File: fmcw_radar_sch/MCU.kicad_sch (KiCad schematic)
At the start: 39 parts, among them J1 2x5 1.27mm, J2 Conn_01x04_Pin, J3 Conn_01x07_Pin, J4 Conn_01x05_Pin, J5 Conn_01x04_Pin, J6 Conn_01x03_Pin, J7 Conn_01x04_Pin, SW1 SW_SPDT, U1 STM32F103C8T6, Y1 HC-49US 16MHZ THT

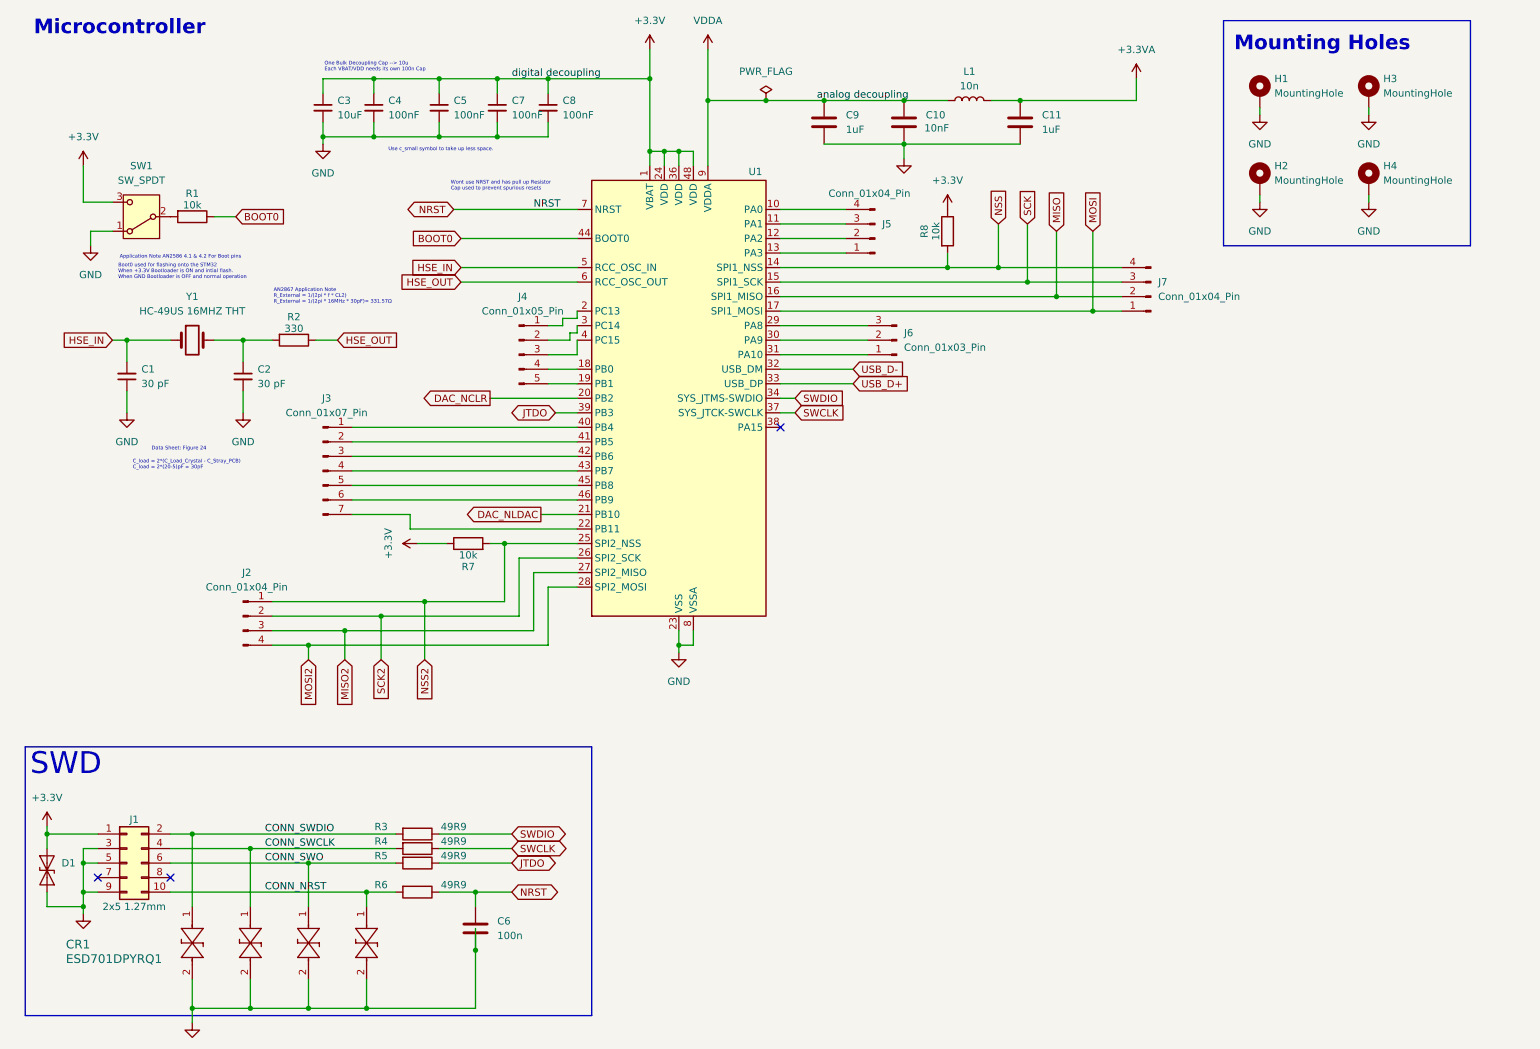
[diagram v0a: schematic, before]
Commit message: changes
changes
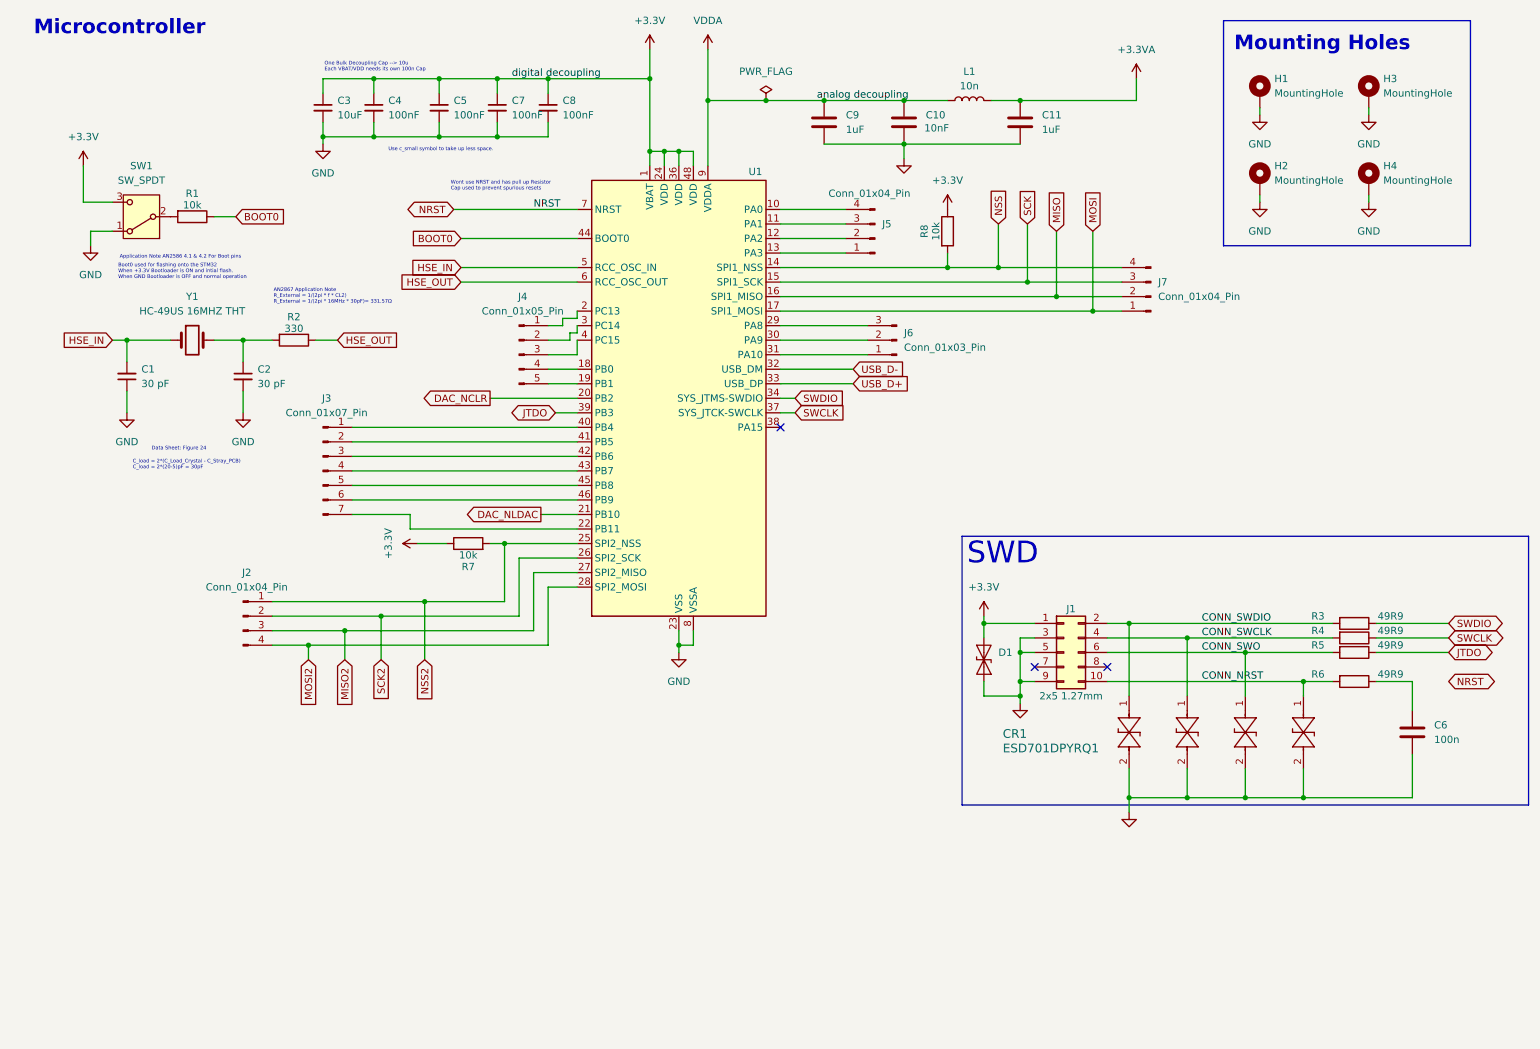
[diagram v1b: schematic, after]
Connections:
- net NRST: no longer C6.1, R6.1
- new net: C6.1, R6.1
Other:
- moved on the sheet: C6, CR1, D1, J1, R3, R4, R5, R6
